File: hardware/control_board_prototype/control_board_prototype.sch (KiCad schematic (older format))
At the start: 14 parts

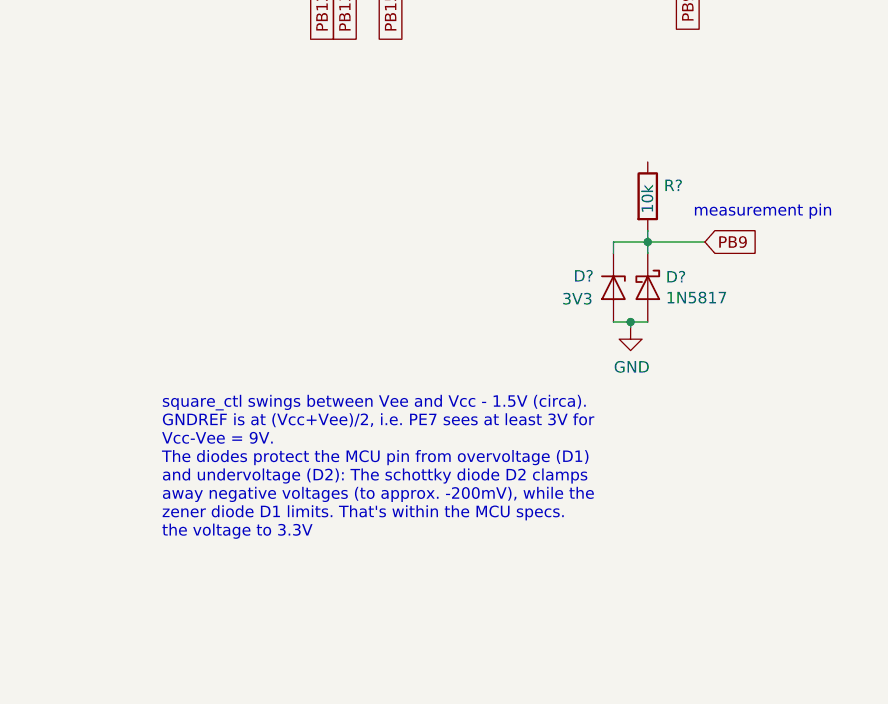
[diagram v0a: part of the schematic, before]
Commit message: put measurement clamping circuitry on the voice board
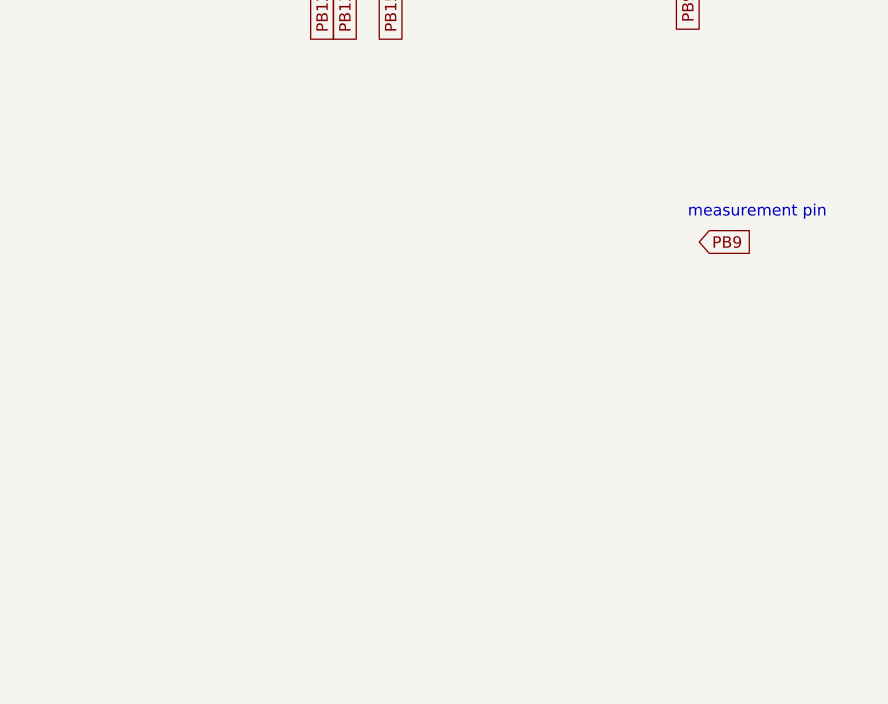
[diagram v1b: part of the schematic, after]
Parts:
- removed D?: 1N5817, Diode_THT:D_DO-41_SOD81_P10.16mm_Horizontal, symbol Diode:1N5817
- removed D?: 3V3, symbol Device:D_Zener
- removed R?: 10k, symbol Device:R
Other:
- note removed: "square_ctl swings between Vee and Vcc - 1.5V (circa).\nGNDREF is at (Vcc+Vee)/2, i.e. PE7 sees at least 3V for\nVcc-Vee = 9V.\nThe diodes protect the MCU pin from overvoltage (D1)\nand undervoltage (D2): The schottky diode D2 clamps\naway negative voltages (to approx. -200mV), while the\nzener diode D1 limits. That's within the MCU specs.\nthe voltage to 3.3V"
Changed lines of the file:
@@
 EESchema Schematic File Version 4
-LIBS:schem-cache
+LIBS:control_board_prototype-cache
 EELAYER 30 0
 EELAYER END
@@
 Text GLabel 775  6550 1    50   Input ~ 0
 Envelope
-Text Notes 8200 6475 0    50   ~ 0
-square_ctl swings between Vee and Vcc - 1.5V (circa).\nGNDREF is at (Vcc+Vee)/2, i.e. PE7 sees at least 3V for\nVcc-Vee = 9V.\nThe diodes protect the MCU pin from overvoltage (D1)\nand undervoltage (D2): The schottky diode D2 clamps\naway negative voltages (to approx. -200mV), while the\nzener diode D1 limits. That's within the MCU specs.\nthe voltage to 3.3V
-$Comp
-L power:GND #PWR?
-U 1 1 5DC28148
-P 10250 5550
-F 0 "#PWR?" H 10250 5300 50  0001 C CNN
-F 1 "GND" H 10255 5377 50  0000 C CNN
-F 2 "" H 10250 5550 50  0001 C CNN
-F 3 "" H 10250 5550 50  0001 C CNN
-	1    10250 5550
-	1    0    0    -1
-$EndComp
-Wire Wire Line
-	10175 5175 10325 5175
-Wire Wire Line
-	10175 5225 10175 5175
-Wire Wire Line
-	10250 5525 10325 5525
-Connection ~ 10250 5525
-Wire Wire Line
-	10250 5550 10250 5525
-Wire Wire Line
-	10175 5525 10250 5525
-$Comp
-L Device:D_Zener D?
-U 1 1 5D432ACA
-P 10175 5375
-F 0 "D?" V 10125 5200 50  0000 L CNN
-F 1 "3V3" V 10225 5150 50  0000 L CNN
-F 2 "" H 10175 5375 50  0001 C CNN
-F 3 "~" H 10175 5375 50  0001 C CNN
-	1    10175 5375
-	0    1    1    0
-$EndComp
-Text Notes 10525 5075 0    50   ~ 0
+Text Notes 10500 5075 0    50   ~ 0
 measurement pin
-Wire Wire Line
-	10325 5175 10325 5125
-Connection ~ 10325 5175
-Wire Wire Line
-	10575 5175 10325 5175
-Text GLabel 10575 5175 2    50   Input ~ 0
+Text GLabel 10550 5175 2    50   Input ~ 0
 PB9
-Wire Wire Line
-	10325 5225 10325 5175
-$Comp
-L Device:R R?
-U 1 1 5D20E97C
-P 10325 4975
-F 0 "R?" H 10395 5021 50  0000 L CNN
-F 1 "10k" V 10325 4900 50  0000 L CNN
-F 2 "" V 10255 4975 50  0001 C CNN
-F 3 "~" H 10325 4975 50  0001 C CNN
-	1    10325 4975
-	1    0    0    -1
-$EndComp
-$Comp
-L Diode:1N5817 D?
-U 1 1 5D20D972
-P 10325 5375
-F 0 "D?" V 10279 5454 50  0000 L CNN
-F 1 "1N5817" V 10370 5454 50  0000 L CNN
-F 2 "Diode_THT:D_DO-41_SOD81_P10.16mm_Horizontal" H 10325 5200 50  0001 C CNN
-F 3 "http://www.vishay.com/docs/88525/1n5817.pdf" H 10325 5375 50  0001 C CNN
-	1    10325 5375
-	0    1    1    0
-$EndComp
 Wire Notes Line
 	8150 625  11050 625

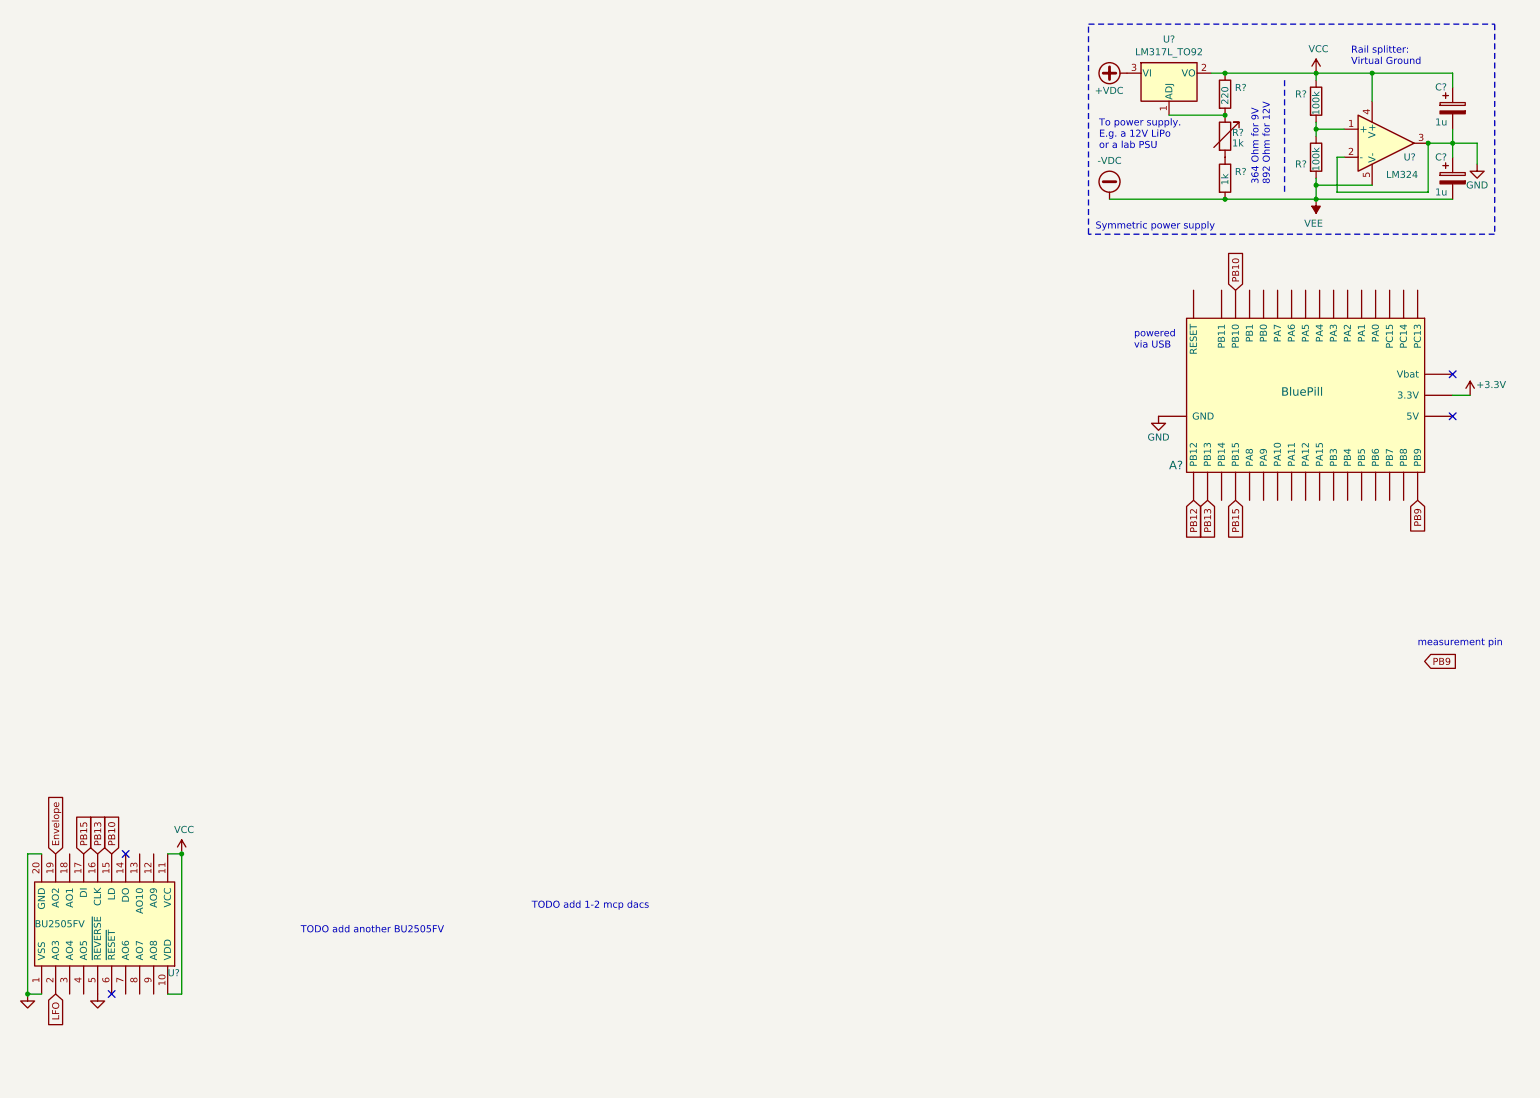
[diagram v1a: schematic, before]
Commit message: control prototype board
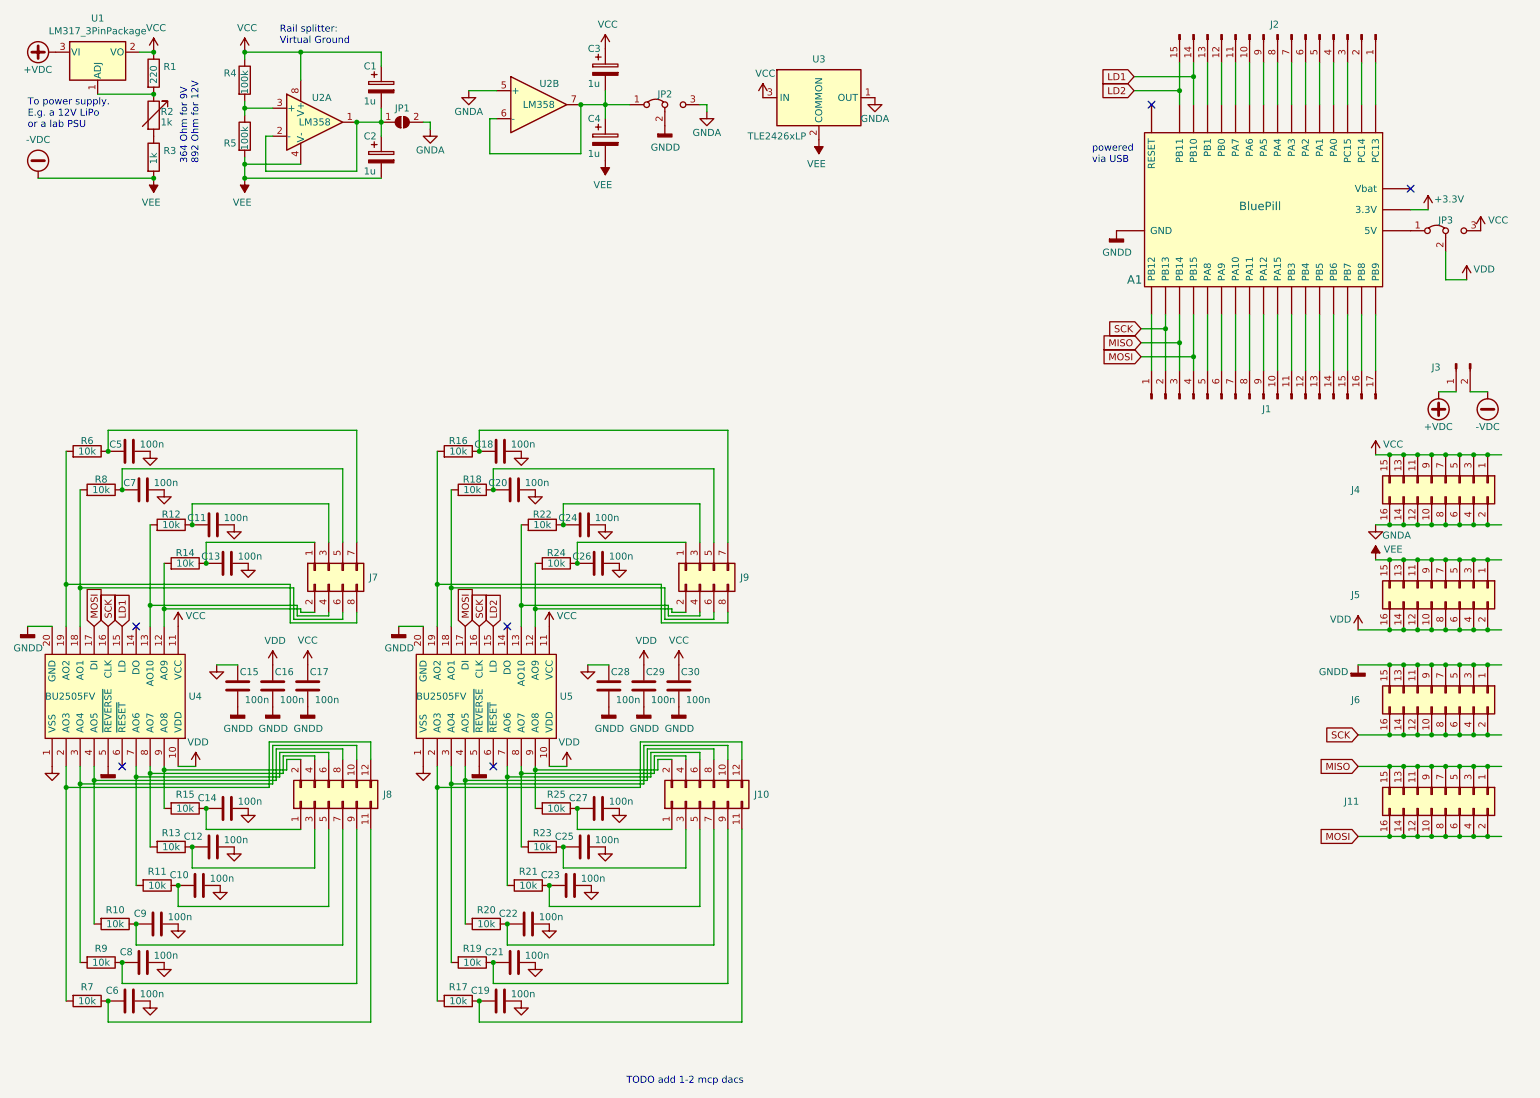
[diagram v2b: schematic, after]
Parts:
- removed U?: LM324, symbol pspice:OPAMP
- removed U?: LM317L_TO92, Package_TO_SOT_THT:TO-92_Inline, symbol Regulator_Linear:LM317L_TO92
- added C10, C11, C12, C13, C14, C15, C16, C17, C18, C19, C20, C21, C22, C23, C24, C25, C26, C27, C28, C29, C30, C5, C6, C7, C8, C9: 100n, Capacitor_SMD:C_0805_2012Metric_Pad1.15x1.40mm_HandSolder, symbol Device:C
- added C3, C4: 1u, Capacitor_THT:CP_Radial_D5.0mm_P2.50mm, symbol Device:CP
- added J1: Conn_01x17_Male, Connector_PinHeader_2.54mm:PinHeader_1x17_P2.54mm_Vertical, symbol Connector:Conn_01x17_Male
- added J10, J8: Conn_02x06_Odd_Even, Connector_PinHeader_2.54mm:PinHeader_2x06_P2.54mm_Vertical, symbol Connector_Generic:Conn_02x06_Odd_Even
- added J11, J4, J5, J6: Conn_02x10_Odd_Even, Connector_PinHeader_2.54mm:PinHeader_2x08_P2.54mm_Vertical, symbol Connector_Generic:Conn_02x08_Odd_Even
- added J2: Conn_01x15_Male, Connector_PinHeader_2.54mm:PinHeader_1x15_P2.54mm_Vertical, symbol Connector:Conn_01x15_Male
- added J3: Conn_01x02_Male, Connector_PinHeader_2.54mm:PinHeader_1x02_P2.54mm_Vertical, symbol Connector:Conn_01x02_Male
- added J7, J9: Conn_02x04_Odd_Even, Connector_PinHeader_2.54mm:PinHeader_2x04_P2.54mm_Vertical, symbol Connector_Generic:Conn_02x04_Odd_Even
- added JP1: SolderJumper_2_Open, windfisch:SolderBridge, symbol Jumper:SolderJumper_2_Open
- added JP2, JP3: Jumper_3_Bridged12, footprints:SolderDipJumper3alt, symbol Jumper:Jumper_3_Bridged12
- added R10, R11, R12, R13, R14, R15, R16, R17, R18, R19, R20, R21, R22, R23, R24, R25, R6, R7, R8, R9: 10k, Resistor_SMD:R_0805_2012Metric_Pad1.15x1.40mm_HandSolder, symbol Device:R
- added U1: LM317_3PinPackage, Package_TO_SOT_THT:TO-220-3_Vertical, symbol Regulator_Linear:LM317_3PinPackage
- added U2: LM358, Package_DIP:DIP-8_W7.62mm, symbol Amplifier_Operational:LM358
- added U3: TLE2426xLP, Package_TO_SOT_THT:TO-92L_Inline, symbol Reference_Voltage:TLE2426xLP
- added U5: BU2505FV, footprints:SSOP20_and_breakout, symbol schematic-symbols:BU2505FV
- A1: renamed from A?; footprint (none) -> footprints:BLUEPILL
- C1, C2: renamed from C?; footprint (none) -> Capacitor_THT:CP_Radial_D5.0mm_P2.50mm
- R1, R3, R4, R5: renamed from R?; footprint (none) -> Resistor_SMD:R_0805_2012Metric_Pad1.15x1.40mm_HandSolder
- R2: renamed from R?; footprint (none) -> Potentiometer_THT:Potentiometer_Bourns_3296W_Vertical
- U4: renamed from U?; footprint Package_SO:SSOP-20_4.4x6.5mm_P0.65mm -> footprints:SSOP20_and_breakout
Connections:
- net +VDC: now also J3.1 (Pin_1), U1.3 (VI)
- net -VDC: now also C4.2, J3.2 (Pin_2), J5.1 (Pin_1), J5.11 (Pin_11), J5.13 (Pin_13), J5.15 (Pin_15), J5.3 (Pin_3), J5.5 (Pin_5), J5.7 (Pin_7), J5.9 (Pin_9), U2.4 (V-), U3.2 (COMMON)
- net VCC: now also C17.1, C3.1, C30.1, J4.1 (Pin_1), J4.11 (Pin_11), J4.13 (Pin_13), J4.15 (Pin_15), J4.3 (Pin_3), J4.5 (Pin_5), J4.7 (Pin_7), J4.9 (Pin_9), JP3.3 (B), U1.2 (VO), U2.8 (V+), U3.3 (IN), U5.11 (VCC); no longer U4.10 (VDD)
- net at R4.2, R5.1: now also U2.3 (+)
- net at R1.2, R2.1: now also U1.1 (ADJ)
- net at U4.12 (AO9): now also J7.2 (Pin_2), R14.2
- net at U4.13 (AO10): now also J7.4 (Pin_4), R12.2
- net at U4.18 (AO1): now also J7.6 (Pin_6), R8.2
- net at U4.3 (AO4): now also J8.10 (Pin_10), R9.2
- net at U4.4 (AO5): now also J8.8 (Pin_8), R10.2
- net at U4.7 (AO6): now also J8.6 (Pin_6), R11.2
- net at U4.8 (AO7): now also J8.4 (Pin_4), R13.2
- net at U4.9 (AO8): now also J8.2 (Pin_2), R15.2
- net at A1.5V: now also JP3.1 (A)
- net at A1.PA0: now also J2.4 (Pin_4)
- net at A1.PA1: now also J2.5 (Pin_5)
- net at A1.PA10: now also J1.7 (Pin_7)
- net at A1.PA11: now also J1.8 (Pin_8)
- net at A1.PA12: now also J1.9 (Pin_9)
- net at A1.PA15: now also J1.10 (Pin_10)
- net at A1.PA2: now also J2.6 (Pin_6)
- net at A1.PA3: now also J2.7 (Pin_7)
- net at A1.PA4: now also J2.8 (Pin_8)
- net at A1.PA5: now also J2.9 (Pin_9)
- net at A1.PA6: now also J2.10 (Pin_10)
- net at A1.PA7: now also J2.11 (Pin_11)
- net at A1.PA8: now also J1.5 (Pin_5)
- net at A1.PA9: now also J1.6 (Pin_6)
- net at A1.PB0: now also J2.12 (Pin_12)
- net at A1.PB1: now also J2.13 (Pin_13)
- net LD2: now reaches A1.PB11
- net LD2: now also J2.15 (Pin_15), U5.15 (LD)
- net MISO: now reaches A1.PB14
- net MISO: now also J1.3 (Pin_3), J11.1 (Pin_1), J11.11 (Pin_11), J11.13 (Pin_13), J11.15 (Pin_15), J11.3 (Pin_3), J11.5 (Pin_5), J11.7 (Pin_7), J11.9 (Pin_9)
- net at A1.PB3: now also J1.11 (Pin_11)
- net at A1.PB4: now also J1.12 (Pin_12)
- net at A1.PB5: now also J1.13 (Pin_13)
- net at A1.PB6: now also J1.14 (Pin_14)
- net at A1.PB7: now also J1.15 (Pin_15)
- net at A1.PB8: now also J1.16 (Pin_16)
- net at A1.PC13: now also J2.1 (Pin_1)
- net at A1.PC14: now also J2.2 (Pin_2)
- net at A1.PC15: now also J2.3 (Pin_3)
- net Envelope: no longer names the net of U4.19 (AO2)
- net Envelope: now also J7.8 (Pin_8), R6.2
- net GND renamed GNDD
- net GNDD: now also C15.2, C16.2, C17.2, C28.2, C29.2, C30.2, J6.1 (Pin_1), J6.11 (Pin_11), J6.13 (Pin_13), J6.15 (Pin_15), J6.3 (Pin_3), J6.5 (Pin_5), J6.7 (Pin_7), J6.9 (Pin_9), JP2.2 (C), U5.20 (GND), U5.5 (~REVERSE); no longer C1.2, C2.1, U4.1 (VSS)
- net LFO: no longer names the net of U4.2 (AO3)
- net LFO: now also J8.12 (Pin_12), R7.2
- net PB10 renamed LD1
- net LD1: now also J2.14 (Pin_14)
- net PB12: no longer names the net of A1.PB12
- net PB12: now also J1.1 (Pin_1)
- net PB13 renamed SCK
- net SCK: now also J1.2 (Pin_2), J6.10 (Pin_10), J6.12 (Pin_12), J6.14 (Pin_14), J6.16 (Pin_16), J6.2 (Pin_2), J6.4 (Pin_4), J6.6 (Pin_6), J6.8 (Pin_8), U5.16 (CLK)
- net PB15 renamed MOSI
- net MOSI: now also J1.4 (Pin_4), J11.10 (Pin_10), J11.12 (Pin_12), J11.14 (Pin_14), J11.16 (Pin_16), J11.2 (Pin_2), J11.4 (Pin_4), J11.6 (Pin_6), J11.8 (Pin_8), U5.17 (DI)
- net PB9: no longer names the net of A1.PB9
- net PB9: now also J1.17 (Pin_17)
- new net: C1.2, C2.1, JP1.1 (A), U2.1, U2.2 (-)
- new net: J9.2 (Pin_2), R24.2, U5.12 (AO9)
- new net: J9.4 (Pin_4), R22.2, U5.13 (AO10)
- new net: J9.6 (Pin_6), R18.2, U5.18 (AO1)
- new net: J9.8 (Pin_8), R16.2, U5.19 (AO2)
- new net: J10.12 (Pin_12), R17.2, U5.2 (AO3)
- new net: J10.10 (Pin_10), R19.2, U5.3 (AO4)
- new net: J10.8 (Pin_8), R20.2, U5.4 (AO5)
- new net: J10.6 (Pin_6), R21.2, U5.7 (AO6)
- new net: J10.4 (Pin_4), R23.2, U5.8 (AO7)
- new net: J10.2 (Pin_2), R25.2, U5.9 (AO8)
- new net: C27.1, J10.1 (Pin_1), R25.1
- new net: C19.1, J10.11 (Pin_11), R17.1
- new net: C25.1, J10.3 (Pin_3), R23.1
- new net: C23.1, J10.5 (Pin_5), R21.1
- new net: C22.1, J10.7 (Pin_7), R20.1
- new net: C21.1, J10.9 (Pin_9), R19.1
- new net: C26.1, J9.1 (Pin_1), R24.1
- new net: C24.1, J9.3 (Pin_3), R22.1
- new net: C20.1, J9.5 (Pin_5), R18.1
- new net: C18.1, J9.7 (Pin_7), R16.1
- new net: C14.1, J8.1 (Pin_1), R15.1
- new net: C6.1, J8.11 (Pin_11), R7.1
- new net: C12.1, J8.3 (Pin_3), R13.1
- new net: C10.1, J8.5 (Pin_5), R11.1
- new net: C9.1, J8.7 (Pin_7), R10.1
- new net: C8.1, J8.9 (Pin_9), R9.1
- new net: C13.1, J7.1 (Pin_1), R14.1
- new net: C11.1, J7.3 (Pin_3), R12.1
- new net: C7.1, J7.5 (Pin_5), R8.1
- new net: C5.1, J7.7 (Pin_7), R6.1
- new net: C3.2, C4.1, JP2.1 (A), U2.6 (-), U2.7
- new net GNDA: C10.2, C11.2, C12.2, C13.2, C14.2, C15.1, C18.2, C19.2, C20.2, C21.2, C22.2, C23.2, C24.2, C25.2, C26.2, C27.2, C28.1, C5.2, C6.2, C7.2, C8.2, C9.2, J4.10 (Pin_10), J4.12 (Pin_12), J4.14 (Pin_14), J4.16 (Pin_16), J4.2 (Pin_2), J4.4 (Pin_4), J4.6 (Pin_6), J4.8 (Pin_8), JP1.2 (B), JP2.3 (B), U2.5 (+), U3.1 (OUT), U4.1 (VSS), U5.1 (VSS)
- new net VDD: C16.1, C29.1, J5.10 (Pin_10), J5.12 (Pin_12), J5.14 (Pin_14), J5.16 (Pin_16), J5.2 (Pin_2), J5.4 (Pin_4), J5.6 (Pin_6), J5.8 (Pin_8), JP3.2 (C), U4.10 (VDD), U5.10 (VDD)
- no-connect marks 4 -> 6
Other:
- note removed: "Symmetric power supply"
- note removed: "TODO add another BU2505FV"
- note removed: "measurement pin"
- moved on the sheet: A1, C1, C2, R1, R2, R3, R4, R5, U4

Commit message: move stuff around
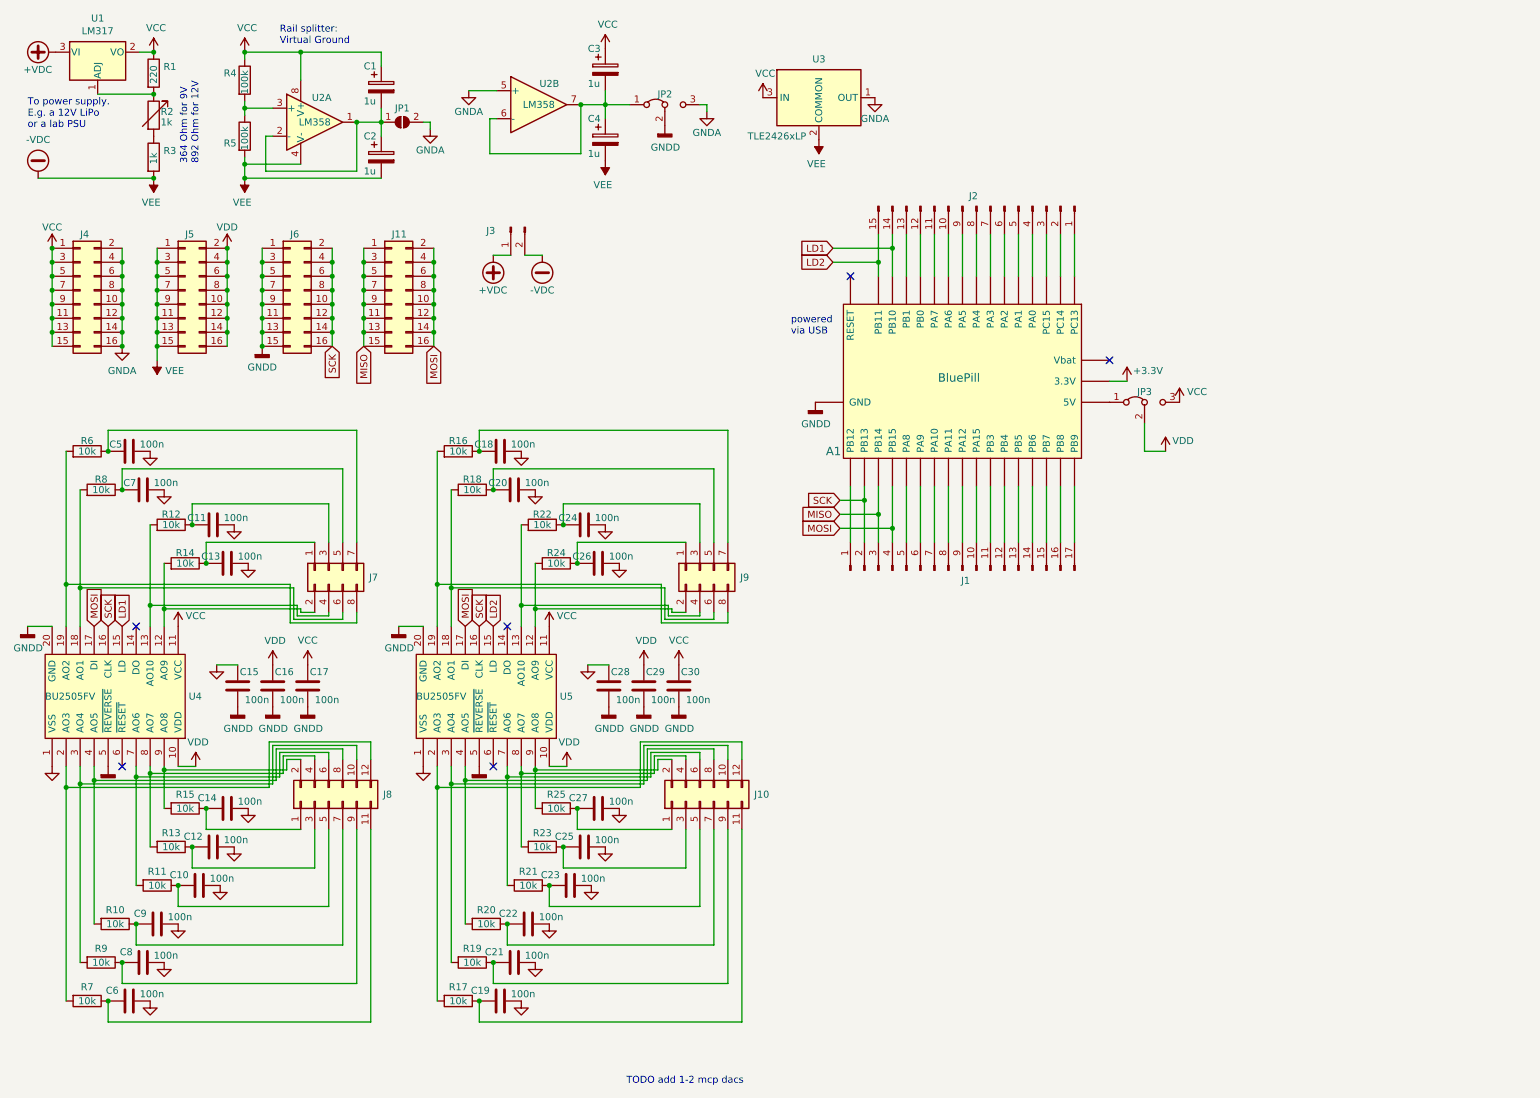
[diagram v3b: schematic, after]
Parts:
- U1: value LM317_3PinPackage -> LM317
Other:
- moved on the sheet: A1, J1, J11, J2, J3, J4, J5, J6, JP3
